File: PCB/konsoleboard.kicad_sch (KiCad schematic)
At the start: 12 parts, among them SW1 SW_Wuerth_450301014042, SW10 SW_Push, SW2 SW_Push, SW3 SW_Wuerth_450301014042, SW5 SW_Push, SW6 SW_Push, SW7 SW_Push, SW8 SW_Push, SW9 SW_Wuerth_450301014042, U3 CR2013-MI2120

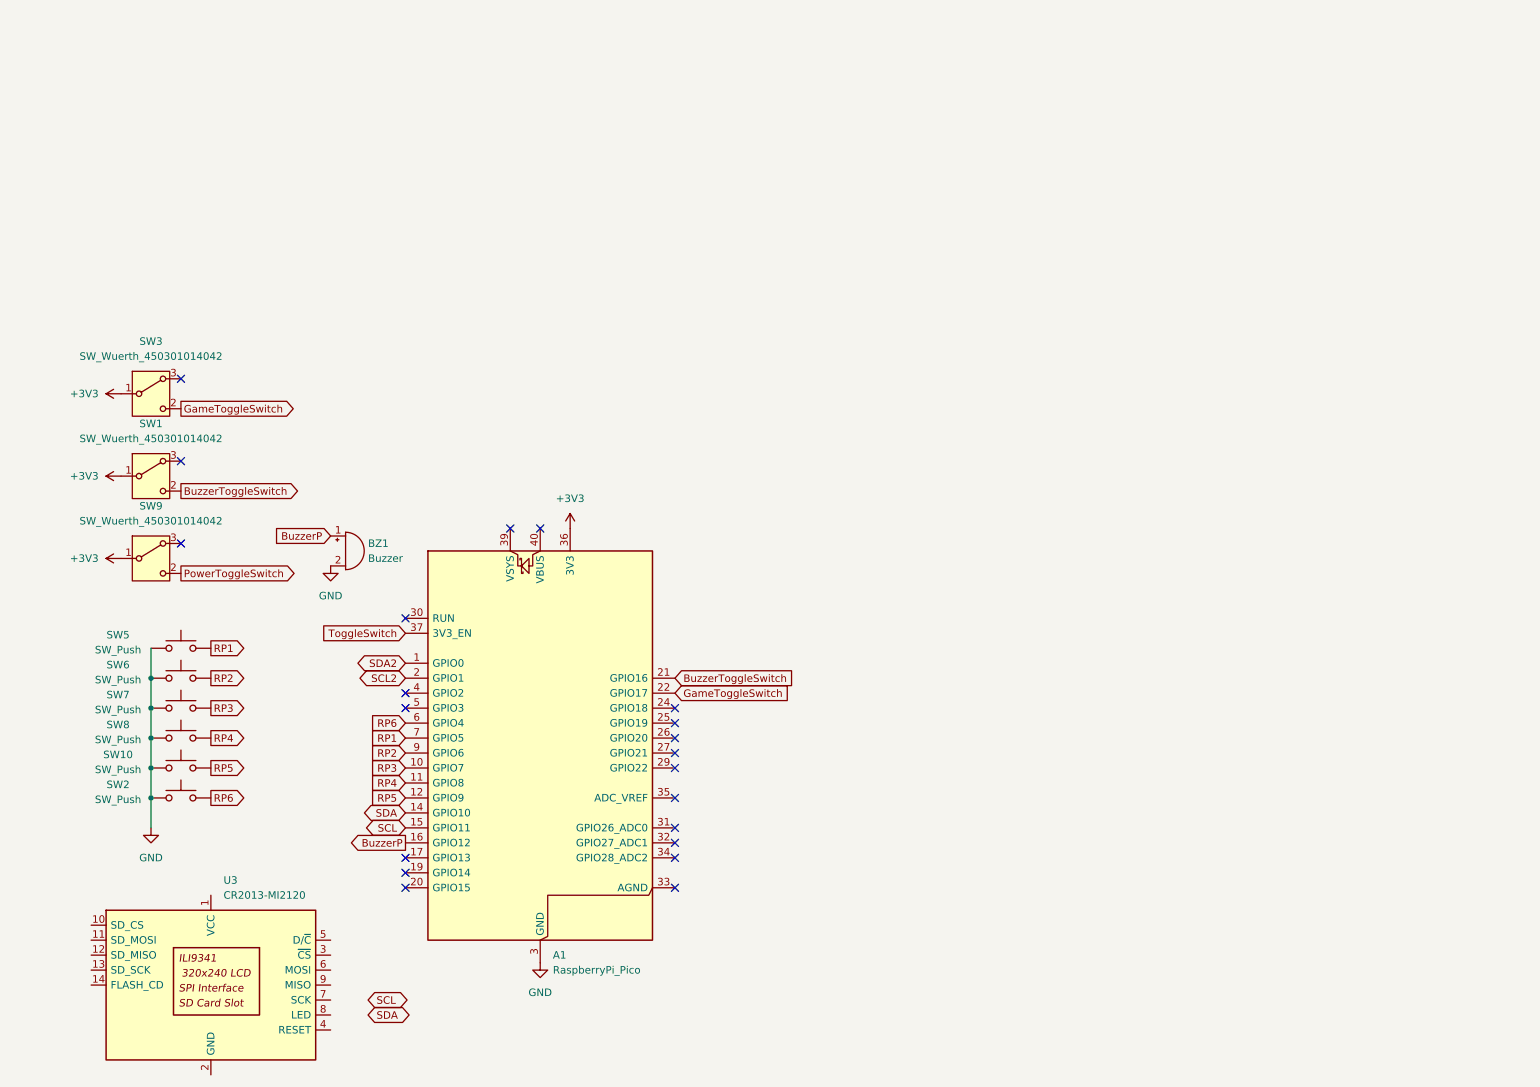
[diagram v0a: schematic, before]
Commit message: Completed the pcb routing
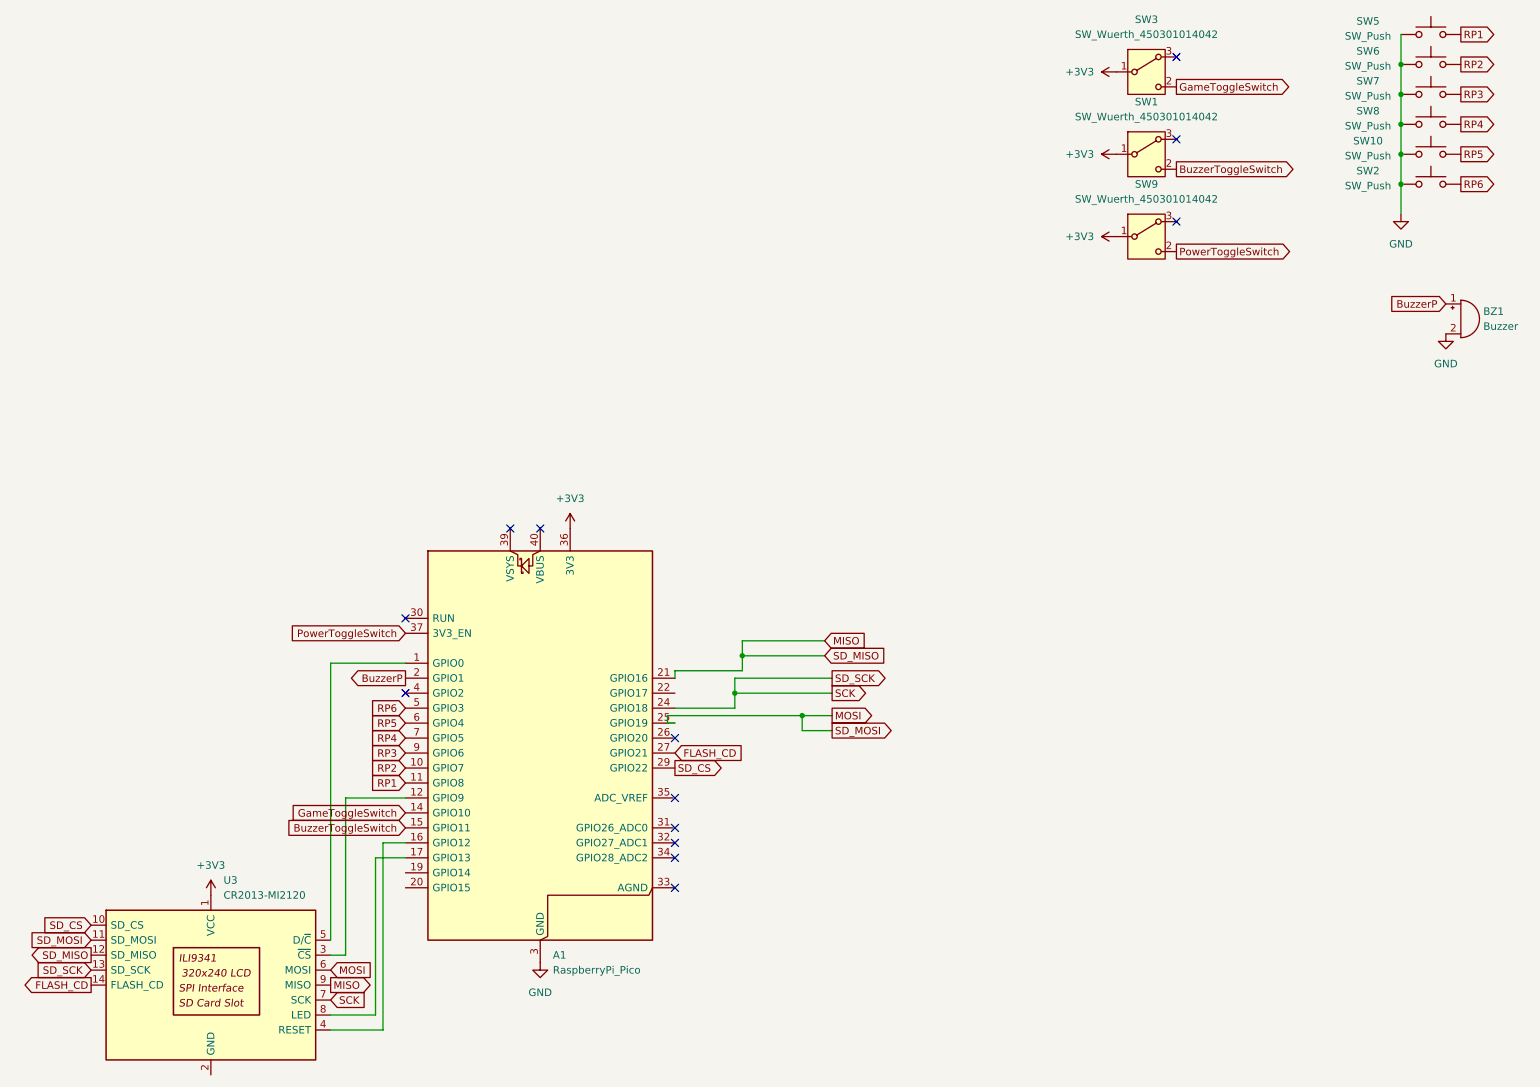
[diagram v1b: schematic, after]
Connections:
- net SCL is gone; now on net BuzzerToggleSwitch: A1.15 (GPIO11)
- net SCL2 is gone; now on net BuzzerP: A1.2 (GPIO1)
- net SDA is gone; now on net GameToggleSwitch: A1.14 (GPIO10)
- net SDA2 is gone; now on an unnamed net: A1.1 (GPIO0)
- net ToggleSwitch is gone; now on net PowerToggleSwitch: A1.37 (3V3_EN)
- net +3V3: now also U3.1 (VCC)
- net BuzzerP: no longer A1.16 (GPIO12)
- net BuzzerToggleSwitch: no longer A1.21 (GPIO16)
- net GameToggleSwitch: no longer A1.22 (GPIO17)
- net RP1: now also A1.11 (GPIO8); no longer A1.7 (GPIO5)
- net RP2: now also A1.10 (GPIO7); no longer A1.9 (GPIO6)
- net RP3: now also A1.9 (GPIO6); no longer A1.10 (GPIO7)
- net RP4: now also A1.7 (GPIO5); no longer A1.11 (GPIO8)
- net RP5: now also A1.6 (GPIO4); no longer A1.12 (GPIO9)
- net RP6: now also A1.5 (GPIO3); no longer A1.6 (GPIO4)
- net SD_CS: now reaches U3.10 (SD_CS)
- net SD_CS: now also A1.29 (GPIO22)
- net MOSI: now reaches U3.11 (SD_MOSI)
- net MOSI: now also A1.25 (GPIO19), U3.6 (MOSI)
- net MISO: now reaches U3.12 (SD_MISO)
- net MISO: now also A1.21 (GPIO16), U3.9 (MISO)
- net SCK: now reaches U3.13 (SD_SCK)
- net SCK: now also A1.24 (GPIO18), U3.7 (SCK)
- net FLASH_CD: now reaches U3.14 (FLASH_CD)
- net FLASH_CD: now also A1.27 (GPIO21)
- net at U3.3 (~{CS}): now also A1.12 (GPIO9)
- net at U3.4 (RESET): now also A1.16 (GPIO12)
- net at U3.8 (LED): now also A1.17 (GPIO13)
- no-connect marks 21 -> 13
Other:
- moved on the sheet: BZ1, SW1, SW10, SW2, SW3, SW5, SW6, SW7, SW8, SW9
